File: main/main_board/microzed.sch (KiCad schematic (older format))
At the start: 16 parts, among them M1 microzed, U6 AP7361C-25SP-13, X1 microzed

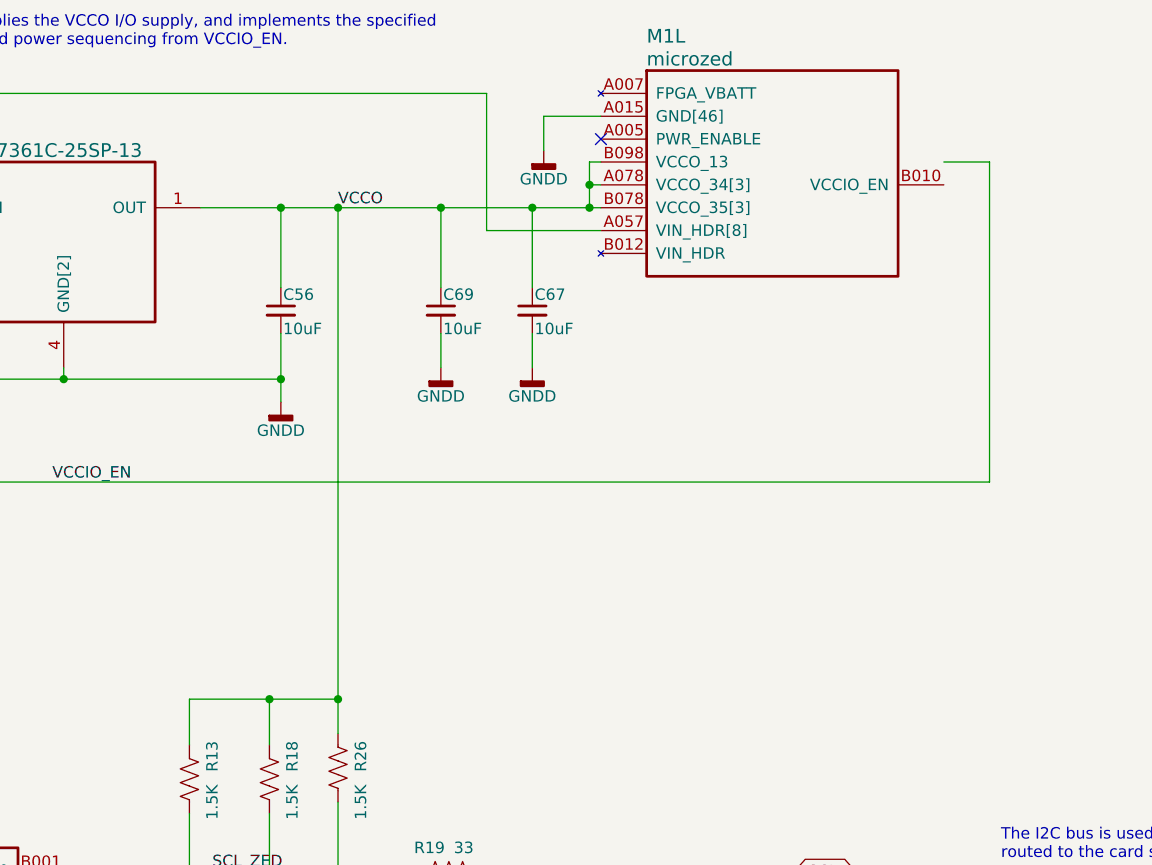
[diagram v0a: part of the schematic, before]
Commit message: Main board is now fully routed and passing DRC. Minor changes related to pin remapping. I2C and one-wire pullups are to OVDD 3.3V, not VCCIO 2.5V. Changes to supply decoupling and VREF- net in reference.sch, suggested by routing.
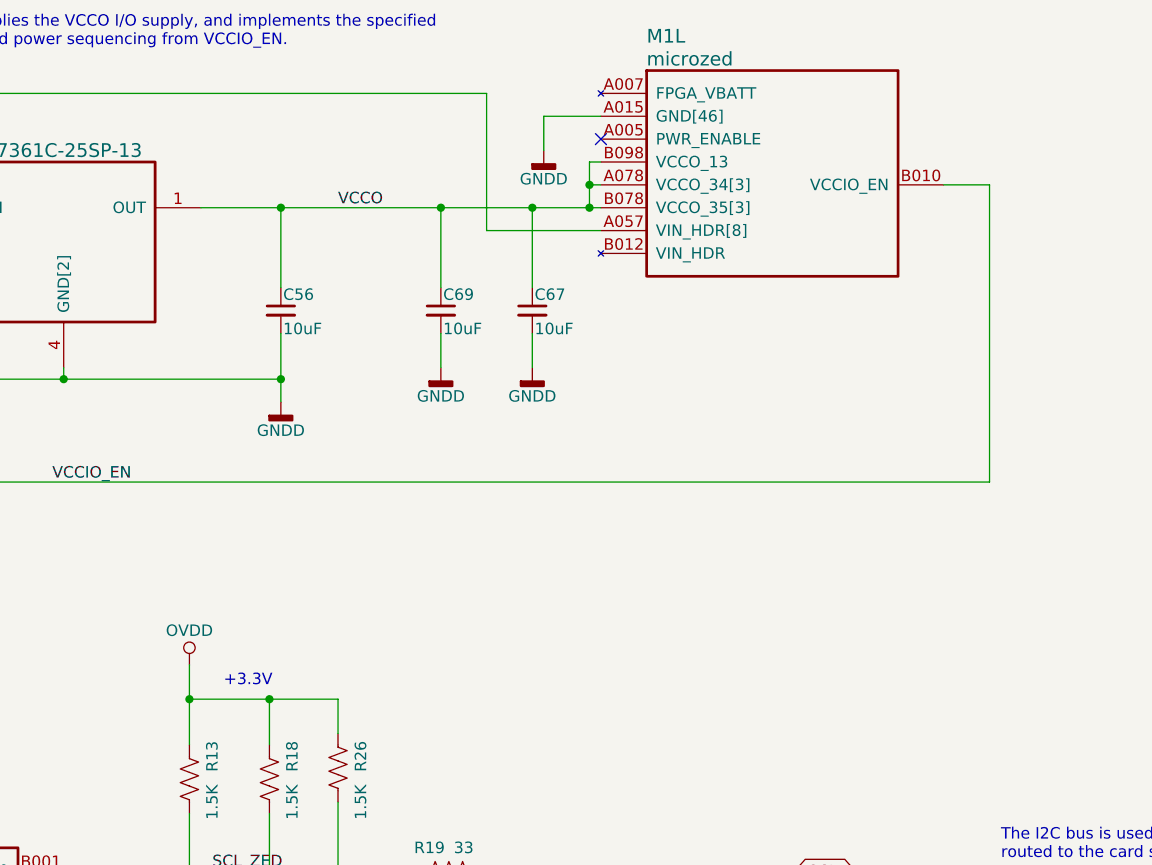
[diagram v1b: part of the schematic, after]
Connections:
- net VCCIO_EN: now also X1.B010 (VCCIO_EN)
- net VCCO: no longer R13.2, R18.2, R26.2
- new net OVDD: R13.2, R18.2, R26.2
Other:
- note added: "+3.3V"
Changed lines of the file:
@@
 	2200 2250 2200 2700
 Wire Wire Line
-	6850 2150 7050 2150
+	6850 2250 7050 2250
 Wire Wire Line
 	1800 2350 2400 2350
@@
 Wire Wire Line
 	4850 2450 5350 2450
-Wire Wire Line
-	7050 2150 7050 3550
 NoConn ~ 3000 5550
 NoConn ~ 3000 5650
@@
 	3550 4500 3550 4700
 Wire Wire Line
-	3950 2350 4200 2350
-Connection ~ 4200 2350
-Wire Wire Line
-	4200 2350 4650 2350
-Wire Wire Line
 	3900 4700 3900 4500
 Wire Wire Line
@@
 $EndComp
 Wire Wire Line
-	4200 2350 4200 4500
-Wire Wire Line
 	4200 5750 4550 5750
 Wire Wire Line
@@
 	3900 4500 4200 4500
 Connection ~ 3900 4500
-Connection ~ 4200 4500
 Wire Wire Line
 	4200 4500 4200 4650
+Wire Wire Line
+	3950 2350 4650 2350
+$Comp
+L ilemt_input:OVDD #PWR0133
+U 1 1 5F0D8254
+P 3550 4350
+AR Path="/5E525F87/5F0D8254" Ref="#PWR0133"  Part="1"
+AR Path="/5E525FFE/5F0D8254" Ref="#PWR?"  Part="1"
+AR Path="/5E525FC9/5F0D8254" Ref="#PWR?"  Part="1"
+F 0 "#PWR0133" H 3550 4200 50  0001 C CNN
+F 1 "OVDD" H 3550 4500 50  0000 C CNN
+F 2 "" H 3550 4350 50  0001 C CNN
+F 3 "" H 3550 4350 50  0001 C CNN
+	1    3550 4350
+	1    0    0    -1
+$EndComp
+Wire Wire Line
+	3550 4350 3550 4500
+Connection ~ 3550 4500
+Text Notes 3700 4450 0    50   ~ 0
++3.3V
+Wire Wire Line
+	7050 2250 7050 3550
 $EndSCHEMATC
